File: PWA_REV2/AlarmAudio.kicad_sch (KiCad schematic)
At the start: 16 parts, among them J1 DFPlayermini, J601 1X2P 1.25 mm Header, J602 0.100_2Pin, J604 2mm_2Pin

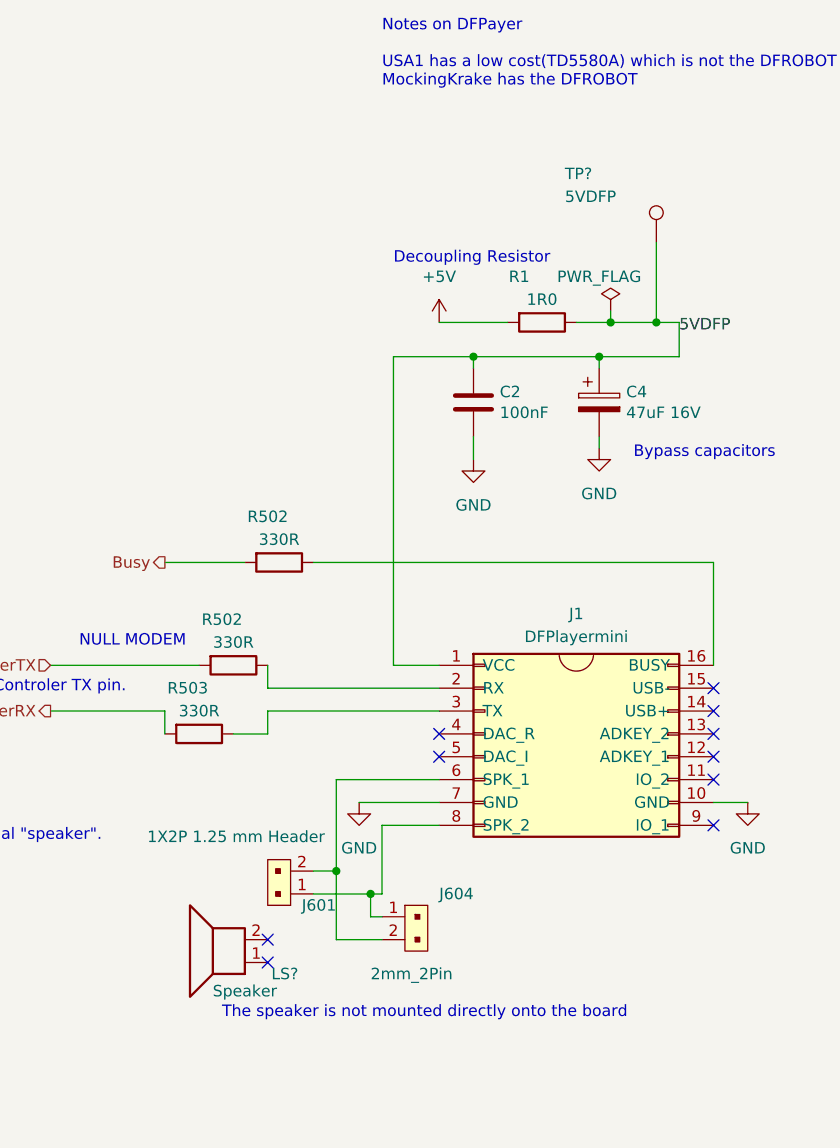
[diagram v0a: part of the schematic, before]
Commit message: Hardware, PWA, Add a Jumper to BOM for J102 so that USB Connector Can Power Krake, issue 312.
:q
q
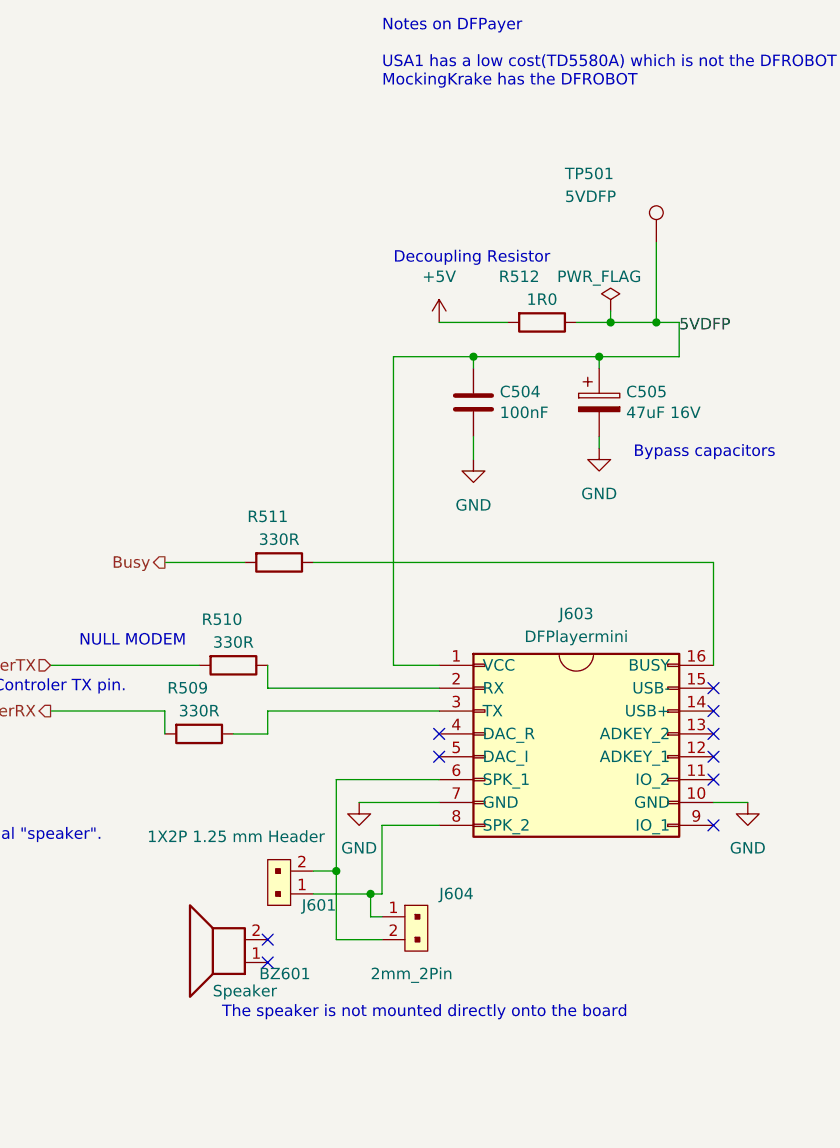
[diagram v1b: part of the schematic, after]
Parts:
- S601: value SWITCH_TACTILE_Projected_12mmx12mm_7.3mm_SPST-NO_0.05A_24V -> SWITCH_TACTILE_Projected_12mmx12mm_7.3mm_SPST-NO_0.05A_24V
- gave numbers to parts that had none: 2
- renumbered C2 to C504, C4 to C505, J1 to J603, R503 to R509, R502 to R510, R502 to R511, R1 to R512

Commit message: Revert "Hardware, PWA, Add a Jumper to BOM for J102 so that USB Connector Can Power Krake, issue 312."
This reverts commit c2819b8ee4999f733f52d823f88f6aefd6456fcc.
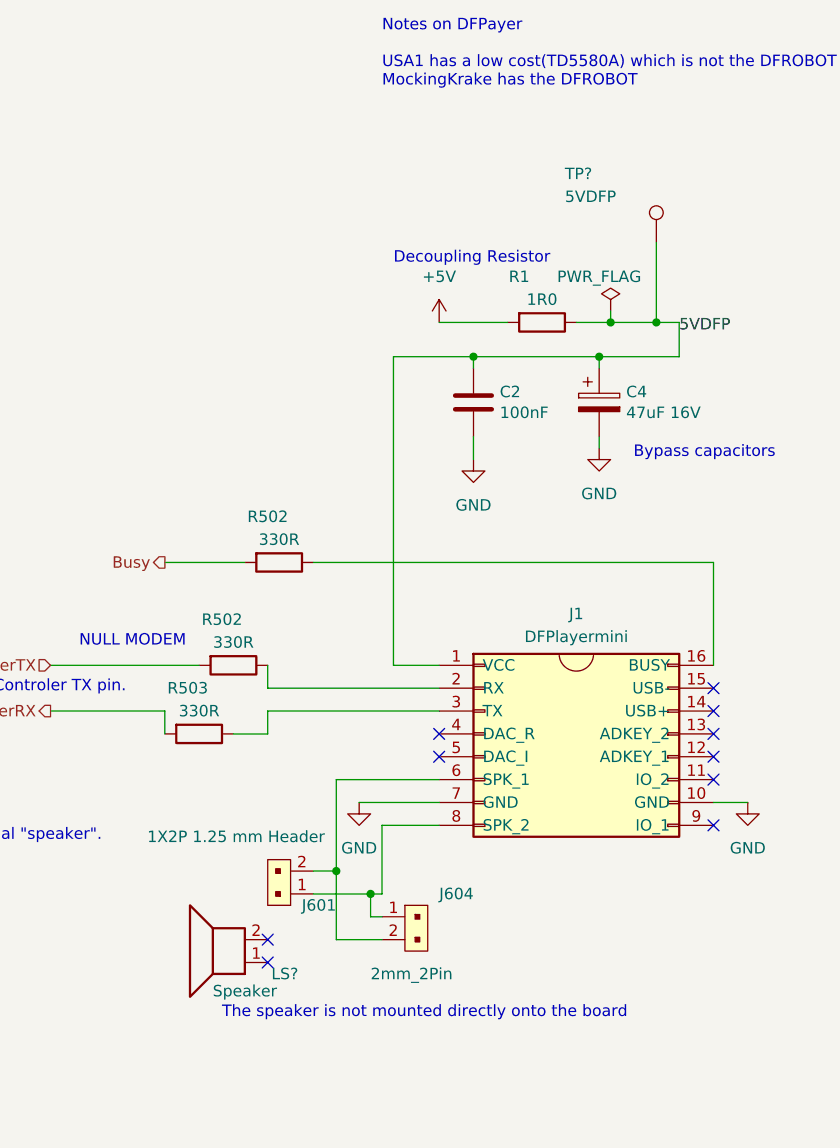
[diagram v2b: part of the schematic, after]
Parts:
- S601: value SWITCH_TACTILE_Projected_12mmx12mm_7.3mm_SPST-NO_0.05A_24V -> SWITCH_TACTILE_Projected_12mmx12mm_7.3mm_SPST-NO_0.05A_24V
- renumbered C504 to C2, C505 to C4, J603 to J1, BZ601 to LS?, R512 to R1, R510 to R502, R511 to R502, R509 to R503, TP501 to TP?
